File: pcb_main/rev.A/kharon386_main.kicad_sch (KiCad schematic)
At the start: 161 parts, among them CON1 CF-CARD-cfcard, J1 USB_B_Micro, J10 COM2, J11 Conn_01x04, J12 ESP, J2 PC104_16, J3 PC104, J4 PJ-322, J5 Conn_02x07_Odd_Even, J6 DB15_Female_HighDensity_Mount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, J7 Mini-DIN-6, J8 COM1, J9 Mini-DIN-6, Q1 BC856, Q2 BC817, SW1 Jumper / Pin header 1x2 Pitch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, SW2 SW_Push, U1 1117-3.3, U10 ST16C554, U11 GD75232PW, U12 MSM5118160F-JS, U13 MSM5118160F-JS, U14 39SF010, U15 TXB0104PW, U16 ESP-12E, U17 ICL7660A, U2 LMR62014, U3 MAX809LEUR, U4 M6117D, U5 74HCT32, U6 74HCT138, U7 74HCT138, U8 GD75232PW, U9 CH340G, X1 14.318 MHz, X2 80 MHz, X3 1.8432 Mhz, Y1 32768 Hz, Y2 12 MHz

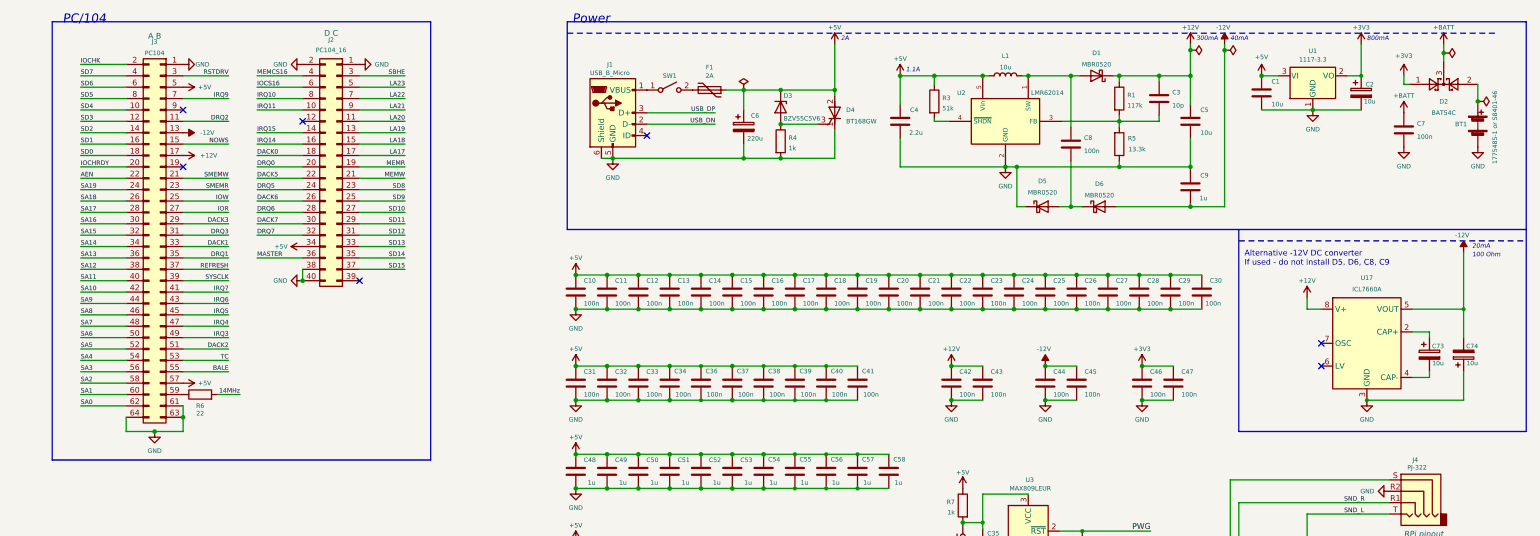
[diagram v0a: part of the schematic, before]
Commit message: wip pcb rev.A
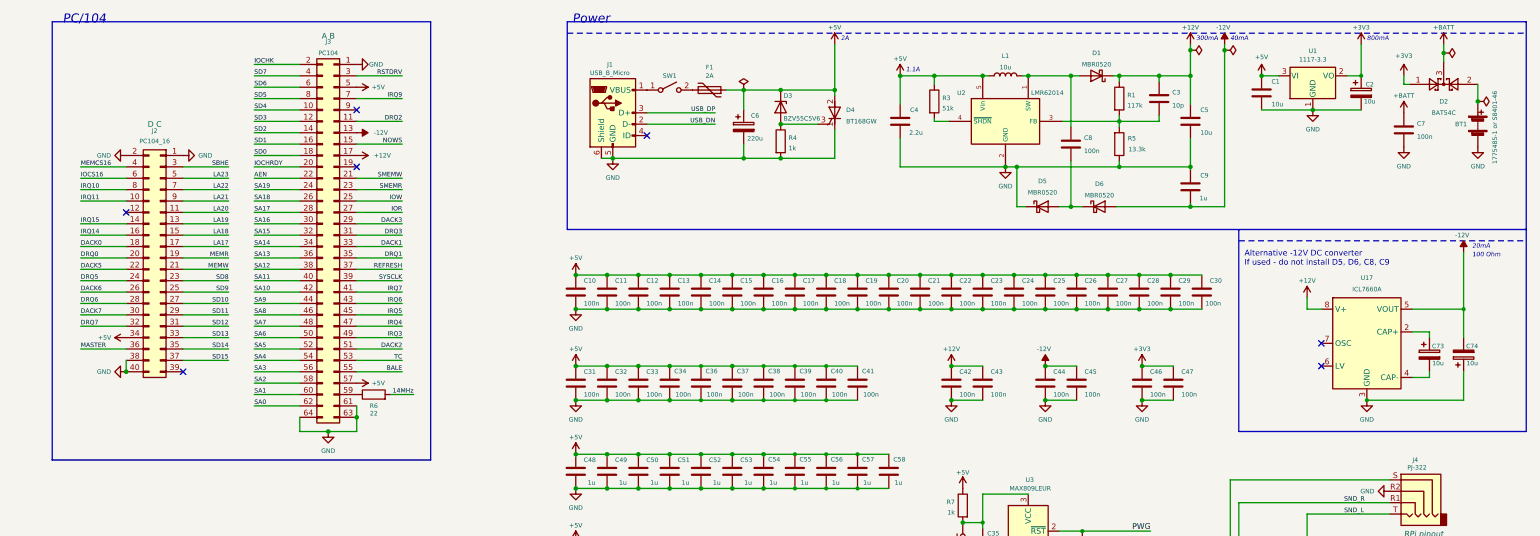
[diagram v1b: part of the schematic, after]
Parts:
- J5: value Conn_02x07_Odd_Even -> Conn_02x08_Odd_Even
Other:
- moved on the sheet: J2, J3, R6
